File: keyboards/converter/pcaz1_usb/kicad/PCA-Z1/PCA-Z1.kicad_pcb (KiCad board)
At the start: 2 copper layers, 161.3 x 19 mm, 3 parts, among them U1 blackpill

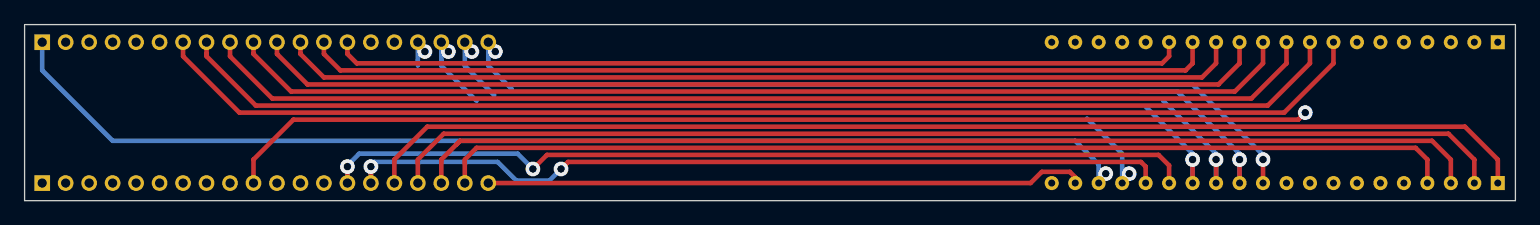
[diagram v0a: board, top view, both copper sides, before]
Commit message: Routed PCB for home etching
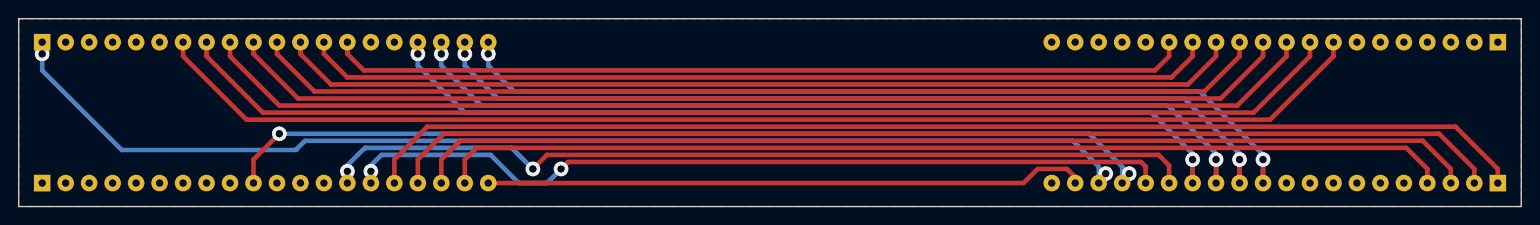
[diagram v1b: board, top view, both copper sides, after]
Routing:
- net MUX_D: track 16.8 -> 97.5 mm
- net MUX_C: track 23.1 -> 97.5 mm
- net MUX_B: track 27.5 -> 97.5 mm
- net LED_CLK: track 128.3 -> 102.3 mm
- net MUX_A: track 95.1 -> 97.5 mm
- net ENC_HALL_A: track 91.3 -> 92.2 mm
- net +5V: track 124.9 -> 125.7 mm, vias 1 -> 2
- net ROW_0: track 92.4 -> 93.1 mm
- net LED_NUM: track 116.3 -> 115.7 mm
- net ENC_LED_V: track 121.7 -> 121.1 mm
- net ENC_LED_H: track 127.4 -> 126.8 mm
- net LED_CAPS: track 110.3 -> 109.7 mm
- net ENC_HALL_B: track 96.8 -> 97.3 mm
- added copper zone on F.Cu, net GND
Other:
- board size 161.3 x 19 mm -> 162.6 x 20.3 mm
